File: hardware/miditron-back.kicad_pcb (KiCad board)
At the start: 2 copper layers, 39.4 x 109.2 mm, 144 parts, among them IC1 SN74AHCT244PW, IC2 LP5012PWR, IC3 DAC8564IAPW, IC4 AD5328BRUZ, IC5 ADP150AUJZ-3.3-R7, J1 Conn_02x06_Odd_Even, J2 Conn_02x06_Odd_Even, J3 Conn_01x10, J32 Debug, J33 Eurorack PWR, J34 Expander, J35 SPI3 Testpoint, J4 Conn_01x12, U1 AT24C256C, U10 MCP6002-xMS, U2 6N137, U3 STM32F401RBTx, U4 OPA4172, U5 TL074, U6 TL074, U7 LM1117-3.3, U8 LM1117-5.0, U9 LM4040DBZ-10, Y1 X50328MSB2GI

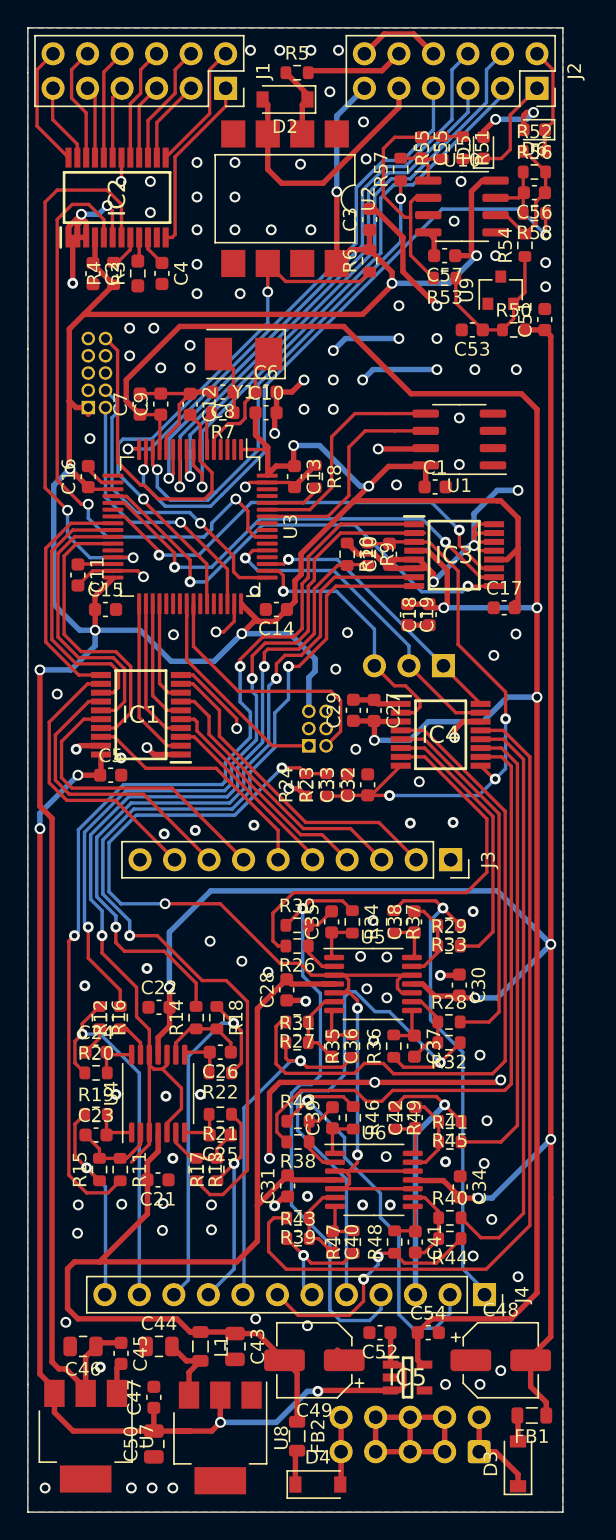
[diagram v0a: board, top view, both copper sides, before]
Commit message: update to kicad 6
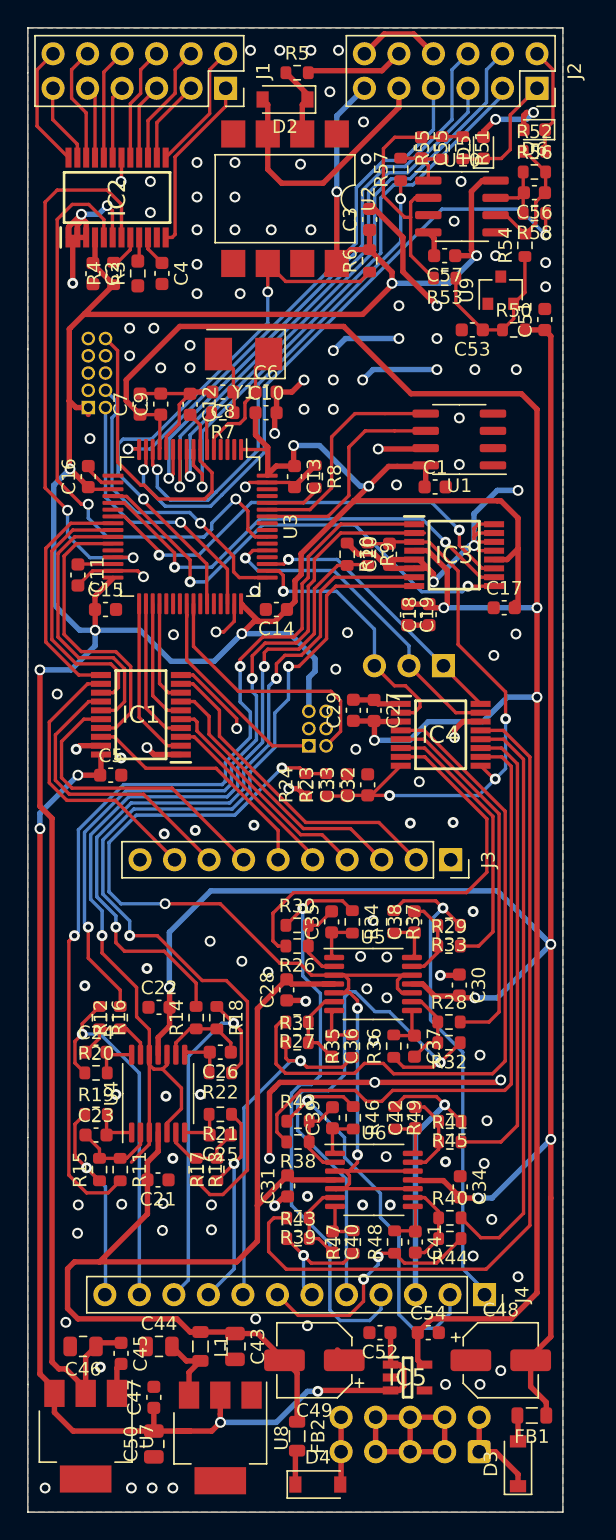
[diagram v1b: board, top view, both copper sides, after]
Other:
- net class Default removed
- net class Power removed
